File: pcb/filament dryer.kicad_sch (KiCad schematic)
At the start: 22 parts, among them J1 Conn_01x02, J2 Screw_Terminal, J3 Conn_01x02, J4 Conn_01x02, J5 Conn_01x02, J6 Screw_Terminal, J7 Conn_01x02, J8 Conn_01x04, Q1 IRLZ44N, Q2 IRLZ44N, U1 SN65HVD230, U2 R-78E5.0-1.0

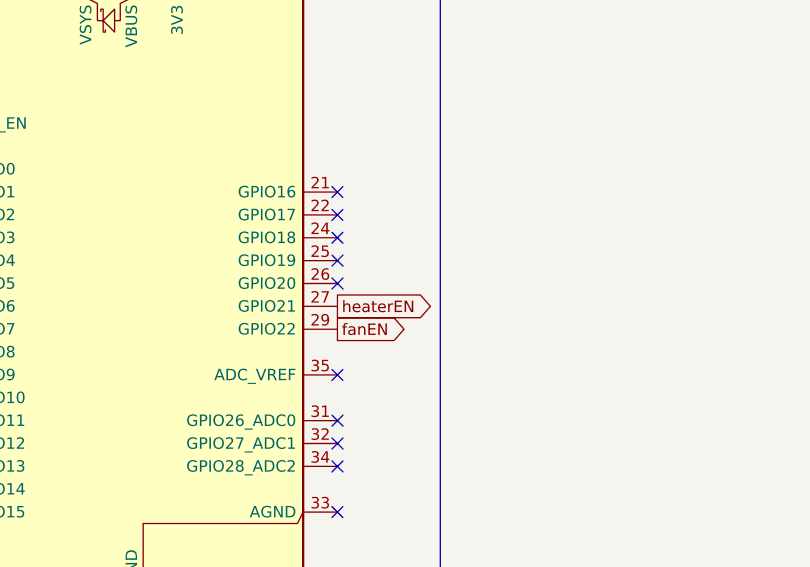
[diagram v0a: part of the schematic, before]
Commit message: pcb update and firmware
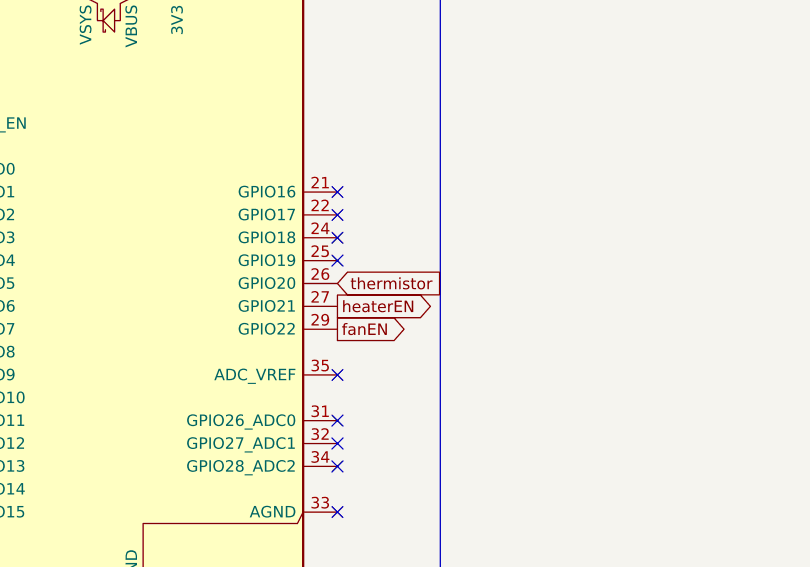
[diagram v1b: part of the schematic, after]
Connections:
- net thermistor: now also A1.26 (GPIO20)
- no-connect marks 25 -> 24
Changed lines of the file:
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@@
-	)
-	(no_connect
-		(at 166.37 59.69)
 	)
 	(no_connect
@@
 			(effects
 				(font
+					(size 1.27 1.27)
+				)
+				(justify left)
+				(hide yes)
+			)
+		)
+	)
+	(global_label "thermistor"
+		(shape input)
+		(at 166.37 59.69 0)
+		(fields_autoplaced yes)
+		(effects
+			(font
+				(size 1.27 1.27)
+			)
+			(justify left)
+		)
+		(property "Intersheetrefs" "${INTERSHEET_REFS}"
+			(at 179.0918 59.69 0)
+			(effects
+				(font
